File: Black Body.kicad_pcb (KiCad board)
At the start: 2 copper layers, 40 x 55.5 mm, 28 parts, among them IC2 MCP96L00T-E_MX, J1 53307-2471, J2 Conn_01x02, J3 Conn_01x03, J4 Conn_02x08_Top_Bottom

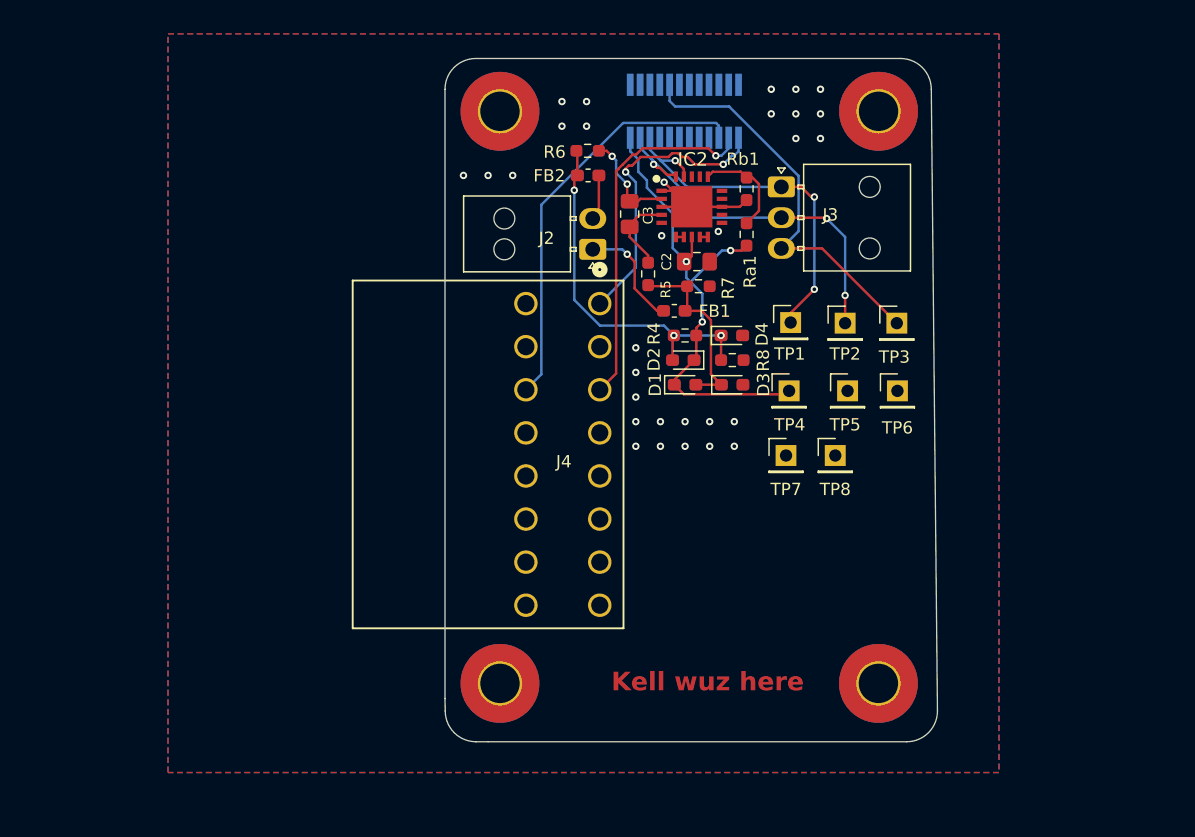
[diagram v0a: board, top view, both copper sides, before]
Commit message: Updated Layout
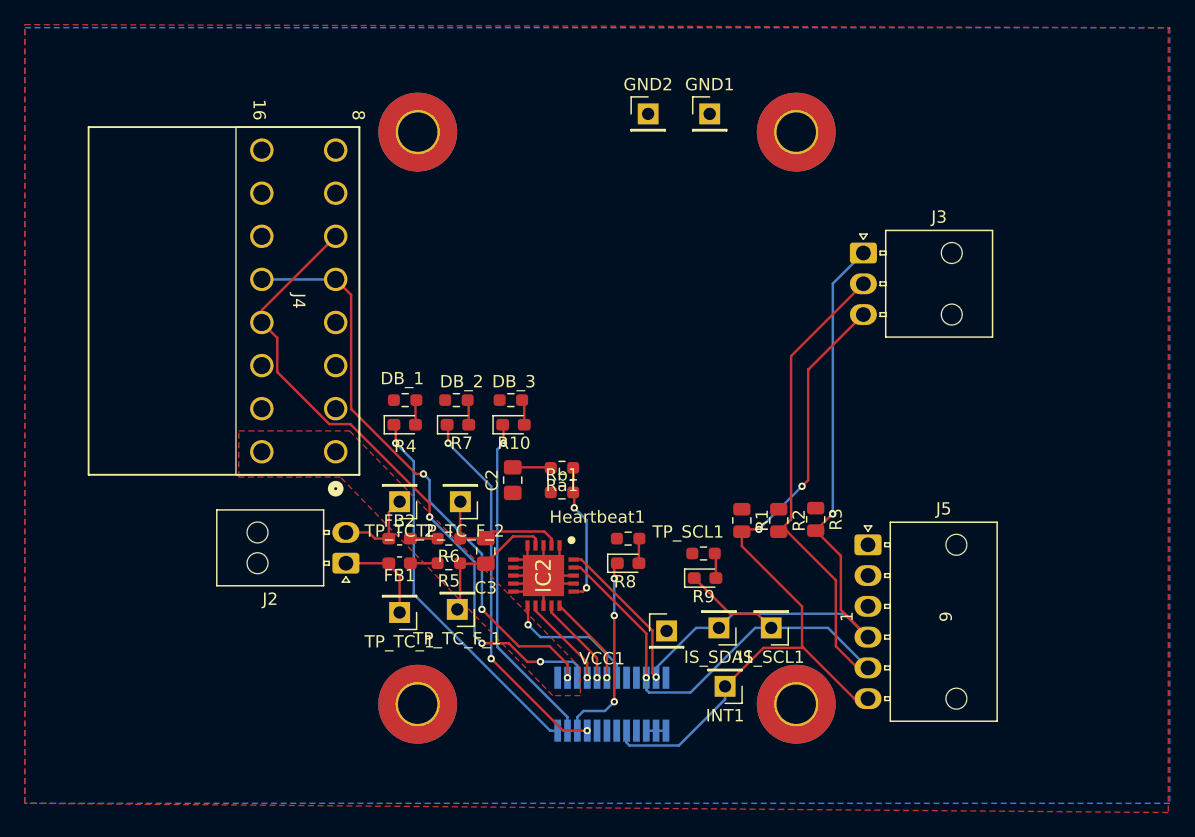
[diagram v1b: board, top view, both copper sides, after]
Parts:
- removed D1, D2, D3, D4: 3V3, Diode_SMD:D_0603_1608Metric_Pad1.05x0.95mm_HandSolder
- removed TP1, TP2, TP3, TP4, TP5, TP6, TP7, TP8: TestPoint, Connector_PinHeader_2.54mm:PinHeader_1x01_P2.54mm_Vertical
- added DB_1: LED, LED_SMD:LED_0603_1608Metric_Pad1.05x0.95mm_HandSolder, F.Cu at (94.2, 94.2)
- added DB_2: LED, LED_SMD:LED_0603_1608Metric_Pad1.05x0.95mm_HandSolder, F.Cu at (98.5, 94.2)
- added DB_3: LED, LED_SMD:LED_0603_1608Metric_Pad1.05x0.95mm_HandSolder, F.Cu at (103.1, 94.2)
- added GND1: TestPoint, Connector_PinHeader_2.54mm:PinHeader_1x01_P2.54mm_Vertical, F.Cu at (119.0, 69.0)
- added GND2: TestPoint, Connector_PinHeader_2.54mm:PinHeader_1x01_P2.54mm_Vertical, F.Cu at (114.0, 69.0)
- added Heartbeat1: LED, LED_SMD:LED_0603_1608Metric_Pad1.05x0.95mm_HandSolder, F.Cu at (112.4, 105.5)
- added INT1: TestPoint, Connector_PinHeader_2.54mm:PinHeader_1x01_P2.54mm_Vertical, F.Cu at (120.2, 115.5)
- added IS_SCL1: TestPoint, Connector_PinHeader_2.54mm:PinHeader_1x01_P2.54mm_Vertical, F.Cu at (124.0, 110.8)
- added IS_SDA1: TestPoint, Connector_PinHeader_2.54mm:PinHeader_1x01_P2.54mm_Vertical, F.Cu at (119.8, 110.8)
- added J5: Conn_01x06, Connector_Molex:Molex_Nano-Fit_105313-xx06_1x06_P2.50mm_Horizontal, F.Cu at (131.9, 104.0)
- added R1: 10k, Resistor_SMD:R_0805_2012Metric, F.Cu at (121.6, 102.0)
- added R10: R, Resistor_SMD:R_0603_1608Metric_Pad0.98x0.95mm_HandSolder, F.Cu at (102.8, 92.2)
- added R2: 1.5k, Resistor_SMD:R_0805_2012Metric, F.Cu at (124.6, 102.0)
- added R3: 1.5k, Resistor_SMD:R_0805_2012Metric, F.Cu at (127.6, 101.9)
- added R9: R, Resistor_SMD:R_0603_1608Metric_Pad0.98x0.95mm_HandSolder, F.Cu at (118.5, 104.7)
- added TP_SCL1: LED, LED_SMD:LED_0603_1608Metric_Pad1.05x0.95mm_HandSolder, F.Cu at (118.6, 106.7)
- added TP_TC_1: TestPoint, Connector_PinHeader_2.54mm:PinHeader_1x01_P2.54mm_Vertical, F.Cu at (93.8, 109.5)
- added TP_TC_2: TestPoint, Connector_PinHeader_2.54mm:PinHeader_1x01_P2.54mm_Vertical, F.Cu at (93.8, 100.5)
- added TP_TC_F_1: TestPoint, Connector_PinHeader_2.54mm:PinHeader_1x01_P2.54mm_Vertical, F.Cu at (98.5, 109.2)
- added TP_TC_F_2: TestPoint, Connector_PinHeader_2.54mm:PinHeader_1x01_P2.54mm_Vertical, F.Cu at (98.8, 100.5)
- added VCC1: TestPoint, Connector_PinHeader_2.54mm:PinHeader_1x01_P2.54mm_Vertical, F.Cu at (115.5, 111.0)
- J3: value Conn_01x03 -> Conn_01x03_Pin
- J4: footprint MX150:CONN_SD-75900-001_2X08_MOL -> UTSVT_Connectors:CONN_SD-75900-001_2X08_MOL
- R4: value 1M -> R
- R7, R8: value 2M -> R
- moved J1 48.5 mm to (111.0, 117.0), turned to 0 degrees
- moved R6 33.5 mm to (97.8, 103.5)
- moved FB2 33.2 mm to (93.8, 103.5), turned to 0 degrees
- moved J2 32.4 mm to (89.5, 105.5)
- moved IC2 32.3 mm to (105.5, 106.5), turned to -90 degrees
- moved FB1 30.3 mm to (93.8, 105.5)
- moved C3 29.8 mm to (100.8, 104.5)
- moved Rb1 28.9 mm to (107.0, 99.8), turned to 0 degrees
- moved R5 28.5 mm to (97.8, 105.5), turned to 180 degrees
- moved J4 24.5 mm to (85.6, 84.2)
- moved Ra1 24.2 mm to (107.0, 97.8), turned to 180 degrees
- moved R4 23.3 mm to (94.3, 92.2), turned to 180 degrees
- moved C2 23.2 mm to (103.0, 98.8), turned to 90 degrees
- moved R7 21.7 mm to (98.4, 92.2)
- moved R8 16.8 mm to (112.4, 103.5)
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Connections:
- net Net-(J1-ADC1_IN7) renamed /INT
- C2 pad 1: +3V3 -> GND
- C2 pad 2: GND -> +3V3
- FB1 pad 2: Net-(D1-A) -> Net-(FB1-Pad2)
- FB2 pad 2: Net-(D2-A) -> Net-(FB2-Pad2)
- IC2 pad 11: unconnected-(IC2-ALERT_1-Pad11) -> /Alert_1
- IC2 pad 12: unconnected-(IC2-ALERT_2-Pad12) -> /Alert_2
- IC2 pad 14: unconnected-(IC2-ALERT_3-Pad14) -> /Alert_3
- IC2 pad 15: unconnected-(IC2-ALERT_4-Pad15) -> /Alert_4
- IC2 pad 19: Net-(IC2-SCL) -> /I2C1_SCL
- IC2 pad 20: Net-(IC2-SDA) -> /I2C1_SDA
- IC2 pad 8: +3V3 -> GND
- J1 pad 12: unconnected-(J1-SPI2_NSS-Pad12) -> /Alert_1
- J1 pad 14: unconnected-(J1-SPI2_MISO-Pad14) -> /Alert_4
- J1 pad 16: unconnected-(J1-SPI2_MOSI-Pad16) -> /Alert_3
- J1 pad 17: unconnected-(J1-SPI1_MOSI-Pad17) -> /DB_Conn_2
- J1 pad 18: unconnected-(J1-SPI2_SCK-Pad18) -> /Alert_2
- J1 pad 19: unconnected-(J1-SPI1_NSS-Pad19) -> /Heartbeat
- J1 pad 20: Net-(J1-CAN_L) -> /CAN_L
- J1 pad 21: unconnected-(J1-SPI1_MISO-Pad21) -> /DB_Conn_3
- J1 pad 22: Net-(J1-CAN_H) -> /CAN_H
- J1 pad 23: unconnected-(J1-SPI1_SCK-Pad23) -> /DB_Conn_1
- J1 pad 24: Net-(J1-+24V_In) -> +24V
- J1 pad 4: Net-(IC2-SDA) -> /I2C1_SDA
- J1 pad 6: Net-(IC2-SCL) -> /I2C1_SCL
- J3 pad 1: Net-(IC2-SCL) -> /I2C1_SDA
- J3 pad 2: Net-(IC2-SDA) -> /I2C1_SCL
- J4 pad 1: Net-(J1-+24V_In) -> +24V
- J4 pad 12: unconnected-(J4-Pin_12-Pad12) -> /CAN_L
- J4 pad 13: unconnected-(J4-Pin_13-Pad13) -> /CAN_H
- J4 pad 5: Net-(J1-CAN_H) -> /CAN_H
- J4 pad 6: Net-(J1-CAN_L) -> /CAN_L
- J4 pad 8: unconnected-(J4-Pin_8-Pad8) -> GND
- J4 pad 9: unconnected-(J4-Pin_9-Pad9) -> +24V
- R4 pad 1: Net-(D2-A) -> Net-(DB_1-A)
- R5 pad 2: Net-(D1-A) -> Net-(FB1-Pad2)
- R6 pad 2: Net-(D2-A) -> Net-(FB2-Pad2)
- R7 pad 1: GND -> Net-(DB_2-A)
- R7 pad 2: Net-(D1-A) -> +3V3
- R8 pad 1: GND -> Net-(Heartbeat1-A)
- R8 pad 2: Net-(D2-A) -> +3V3
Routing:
- net /I2C1_SCL: track 0.00 -> 80.2 mm, vias 0 -> 1
- net /I2C1_SDA: track 0.00 -> 68.2 mm, vias 0 -> 2
- net /CAN_L: track 0.00 -> 53.4 mm, vias 0 -> 3
- net /CAN_H: track 0.00 -> 48.0 mm, vias 0 -> 3
- net +3V3: track 41.1 -> 3.10 mm, vias 3 -> 0
- net Net-(J1-CAN_L): track 33.8 -> 0.00 mm
- net /DB_Conn_1: track 0.00 -> 30.7 mm, vias 0 -> 1
- net /DB_Conn_2: track 0.00 -> 30.7 mm, vias 0 -> 3
- net Net-(IC2-SDA): track 30.6 -> 0.00 mm, vias 3 -> 0
- net Net-(IC2-SCL): track 30.1 -> 0.00 mm, vias 3 -> 0
- net Net-(J1-CAN_H): track 29.6 -> 0.00 mm, vias 1 -> 0
- net Net-(D2-A): track 29.5 -> 0.00 mm, vias 3 -> 0
- net /INT: track 32.7 -> 60.5 mm, vias 0 -> 2
- net /DB_Conn_3: track 0.00 -> 27.4 mm, vias 0 -> 1
- net Net-(J1-+24V_In): track 24.1 -> 0.00 mm, vias 2 -> 0
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- added copper zone on F.Cu, net +24V
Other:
- board outline removed
- board text removed: "Kell wuz here"
